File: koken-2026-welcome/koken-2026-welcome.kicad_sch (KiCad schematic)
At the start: 16 parts, among them J1 USB_C_Receptacle_USB2.0_16P, SW1 SW_Push, U1 CH32V003JxMx, U2 AP7333

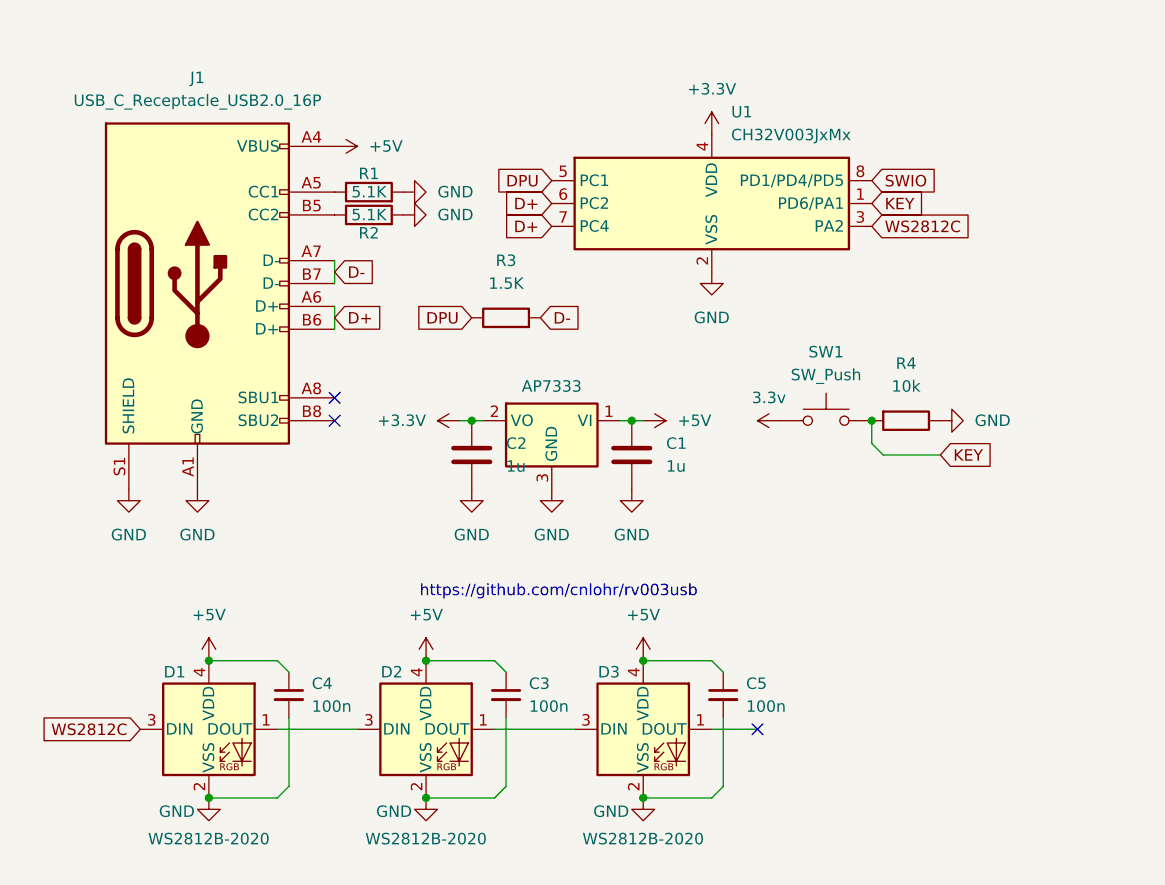
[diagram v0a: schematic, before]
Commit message: 回路図完成
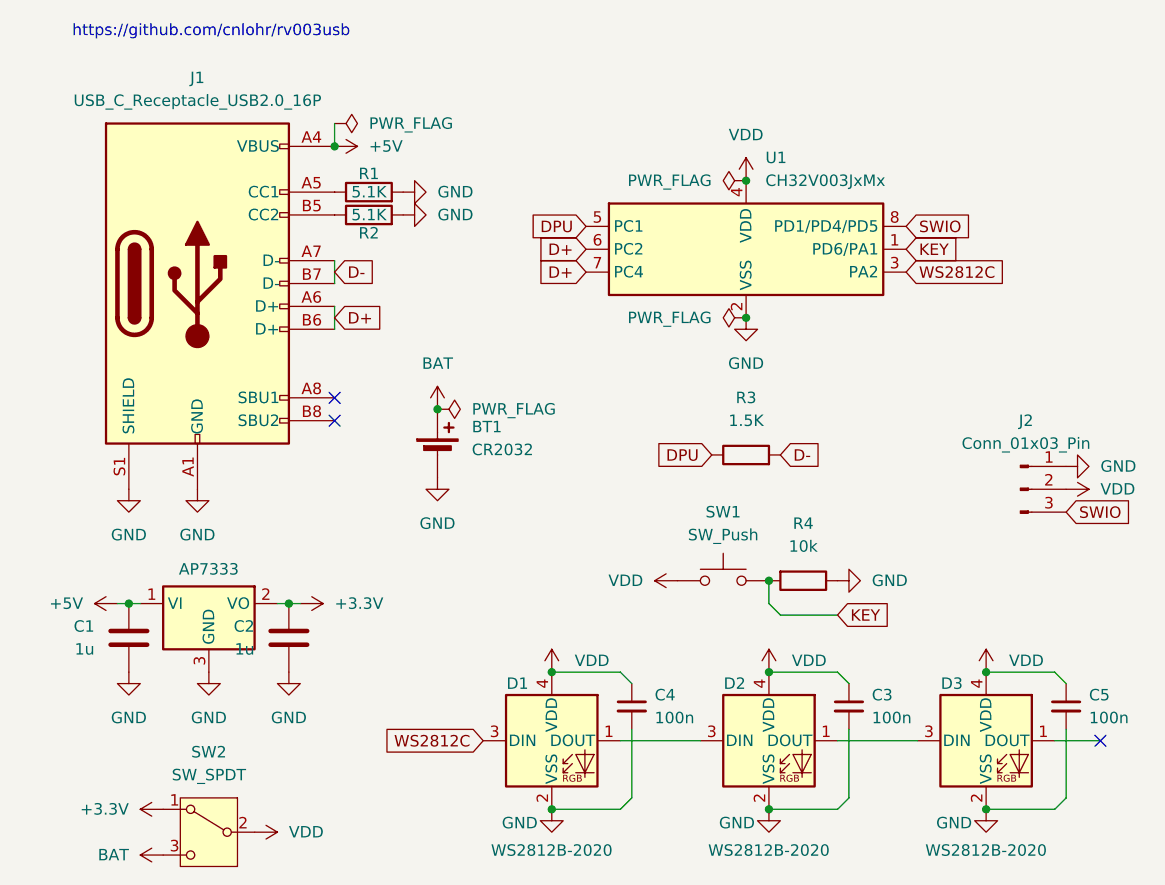
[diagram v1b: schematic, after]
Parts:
- added BT1: CR2032, symbol Device:Battery_Cell
- added J2: Conn_01x03_Pin, symbol Connector:Conn_01x03_Pin
- added SW2: SW_SPDT, symbol Switch:SW_SPDT
- C1, C2, C3, C4, C5: footprint (none) -> Capacitor_SMD:C_0603_1608Metric_Pad1.08x0.95mm_HandSolder
- R1, R2, R3, R4: footprint (none) -> Resistor_SMD:R_0603_1608Metric_Pad0.98x0.95mm_HandSolder
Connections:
- net +3.3V: now also SW2.1 (A); no longer U1.4 (VDD)
- net +5V: no longer C3.1, C4.1, C5.1, D1.4 (VDD), D2.4 (VDD), D3.4 (VDD)
- net GND: now also BT1.2 (-), J2.1 (Pin_1)
- net SWIO: now also J2.3 (Pin_3)
- net 3.3v renamed VDD
- net VDD: now also C3.1, C4.1, C5.1, D1.4 (VDD), D2.4 (VDD), D3.4 (VDD), U1.4 (VDD), J2.2 (Pin_2), SW2.2 (B)
- new net BAT: BT1.1 (+), SW2.3 (C)
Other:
- moved on the sheet: C1, C2, C3, C4, C5, D1, D2, D3, R3, R4, SW1, U1

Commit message: assign footprint
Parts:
- BT1, SW1: footprint (none) -> Library:CherryMX_Red
- J1: footprint (none) -> Connector_USB:USB_C_Receptacle_GCT_USB4105-xx-A_16P_TopMnt_Horizontal
- J2: footprint (none) -> Connector_PinHeader_2.54mm:PinHeader_1x03_P2.54mm_Vertical
- SW2: footprint (none) -> Button_Switch_THT:SW_Slide-03_Wuerth-WS-SLTV_10x2.5x6.4_P2.54mm
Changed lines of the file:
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@@
 			)
 		)
-		(property "Footprint" ""
+		(property "Footprint" "Button_Switch_THT:SW_Slide-03_Wuerth-WS-SLTV_10x2.5x6.4_P2.54mm"
 			(at 55.88 148.59 0)
 			(effects
@@
 			)
 		)
-		(property "Footprint" ""
+		(property "Footprint" "Connector_PinHeader_2.54mm:PinHeader_1x03_P2.54mm_Vertical"
 			(at 146.05 110.49 0)
 			(effects
@@
 			)
 		)
-		(property "Footprint" ""
+		(property "Footprint" "Library:CherryMX_Red"
 			(at 113.03 115.57 0)
 			(effects
@@
 			)
 		)
-		(property "Footprint" ""
+		(property "Footprint" "Connector_USB:USB_C_Receptacle_GCT_USB4105-xx-A_16P_TopMnt_Horizontal"
 			(at 58.42 87.63 0)
 			(effects
@@
 			)
 		)
-		(property "Footprint" ""
+		(property "Footprint" "Library:CherryMX_Red"
 			(at 81.28 105.156 90)
 			(effects

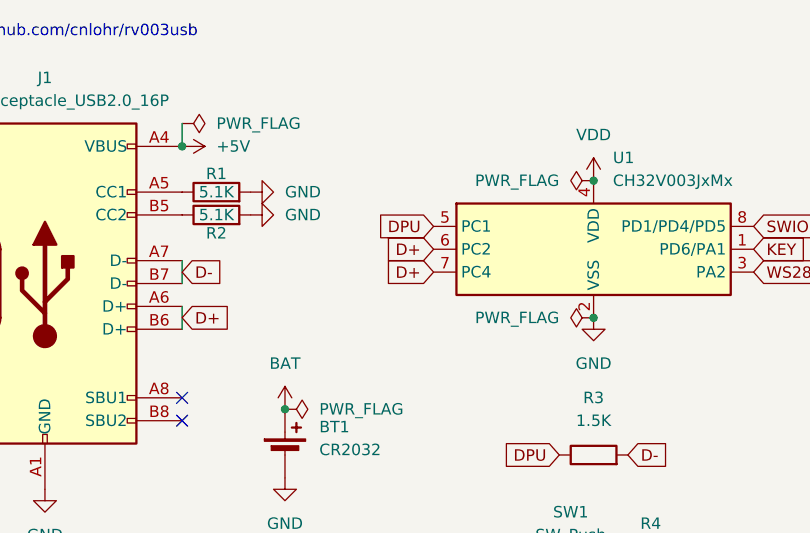
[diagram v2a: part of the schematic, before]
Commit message: fix
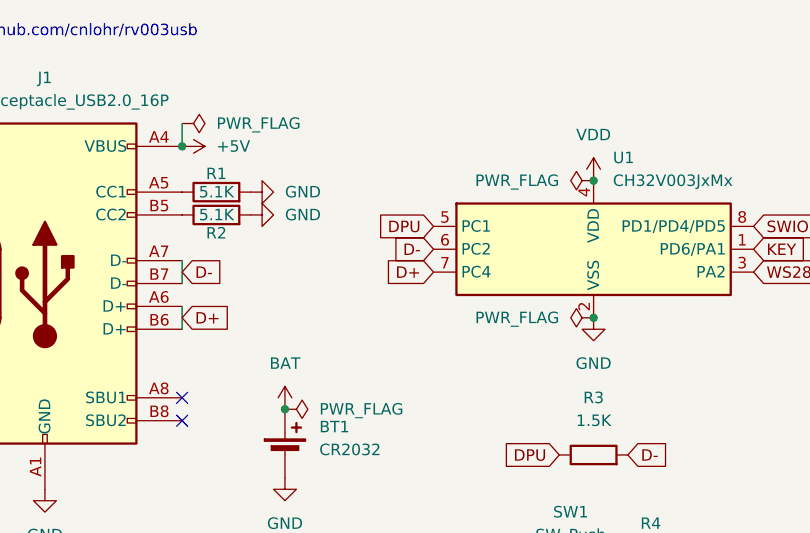
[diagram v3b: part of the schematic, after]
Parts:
- BT1: footprint Library:CherryMX_Red -> Battery:BatteryHolder_MPD_BC2003_1x2032
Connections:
- net D+: no longer U1.6 (PC2)
- net D-: now also U1.6 (PC2)
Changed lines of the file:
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@@
 		)
 	)
-	(global_label "D+"
+	(global_label "D-"
 		(shape input)
 		(at 97.79 83.82 180)
@@
 			)
 		)
-		(property "Footprint" "Library:CherryMX_Red"
+		(property "Footprint" "Battery:BatteryHolder_MPD_BC2003_1x2032"
 			(at 81.28 105.156 90)
 			(effects

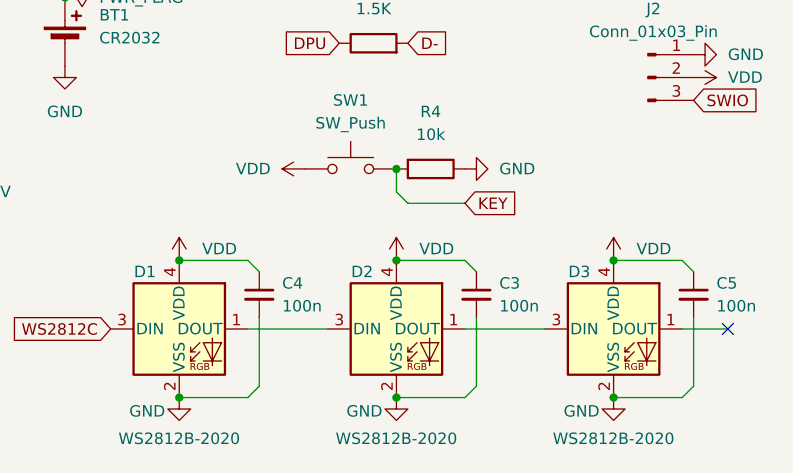
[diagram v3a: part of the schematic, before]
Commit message: -
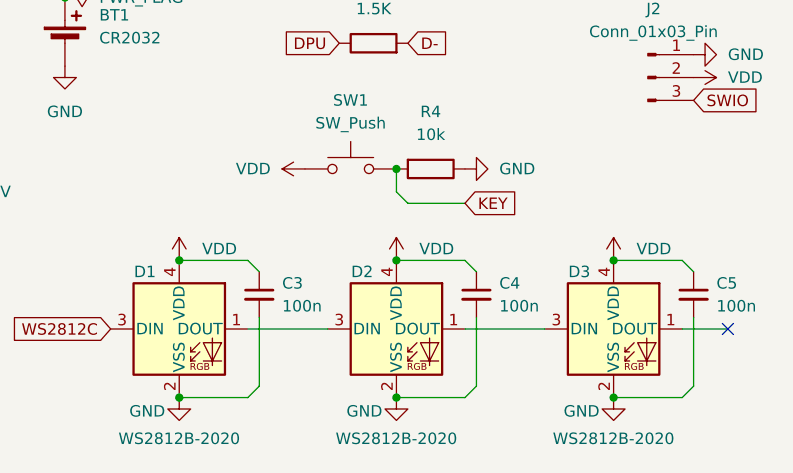
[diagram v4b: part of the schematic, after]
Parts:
- renumbered C4 to C3, C3 to C4
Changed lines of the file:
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@@
 		(dnp no)
 		(fields_autoplaced yes)
-		(property "Reference" "C4"
+		(property "Reference" "C3"
 			(at 105.41 133.3562 0)
 			(effects
@@
 			(project ""
 				(path "/c1514d4b-c430-4cc3-b61b-88eeca3cb740"
-					(reference "C4")
+					(reference "C3")
 					(unit 1)
 				)
@@
 		(dnp no)
 		(fields_autoplaced yes)
-		(property "Reference" "C3"
+		(property "Reference" "C4"
 			(at 129.54 133.3562 0)
 			(effects
@@
 			(project "koken-2026-welcome"
 				(path "/c1514d4b-c430-4cc3-b61b-88eeca3cb740"
-					(reference "C3")
-					(unit 1)
-				)
+					(reference "C4")
+					(unit 1)
+				)
